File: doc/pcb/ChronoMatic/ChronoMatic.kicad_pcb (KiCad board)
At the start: 2 copper layers, 73 x 73.1 mm, 24 parts, among them Q1 Q_Photo_NPN, U1 STM32F030F4Px, Y1 7.3728

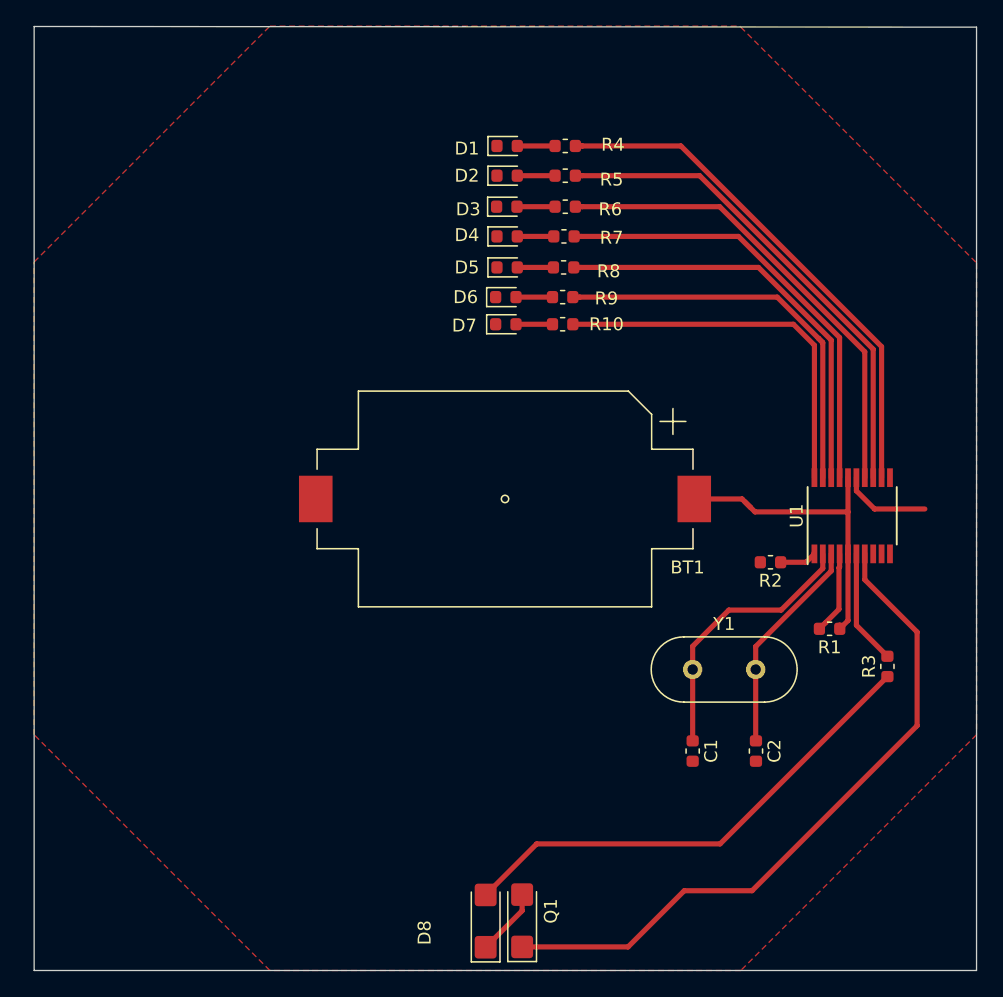
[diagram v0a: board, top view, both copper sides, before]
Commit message: new design
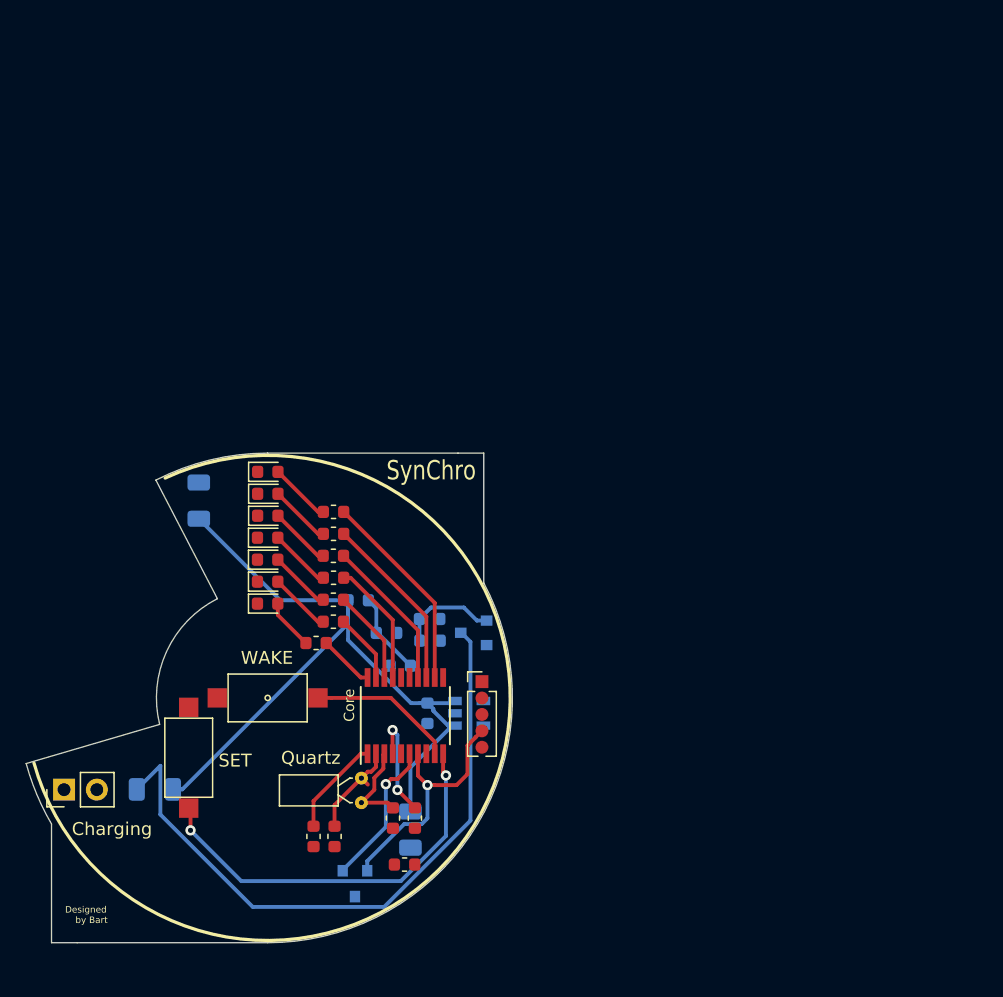
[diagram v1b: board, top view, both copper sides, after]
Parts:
- removed D8: LED, LED_SMD:LED_1806_4516Metric_Castellated
- removed Y1: 7.3728, Crystal:Crystal_HC49-U_Vertical
- added   : Conn_01x05_Female, Connector_PinHeader_1.27mm:PinHeader_1x05_P1.27mm_Vertical, F.Cu at (235.7, 115.0)
- added BT2: Battery_Cell, Resistor_SMD:R_1206_3216Metric, B.Cu at (230.2, 126.5)
- added C3: 10p, Capacitor_SMD:C_0603_1608Metric, F.Cu at (224.3, 127.0)
- added C4: 10p, Capacitor_SMD:C_0603_1608Metric, F.Cu at (228.8, 125.6)
- added C5: 2.2u, Capacitor_SMD:C_0603_1608Metric, B.Cu at (228.3, 111.3)
- added Charging: Charging port, Connector_PinHeader_2.54mm:PinHeader_1x02_P2.54mm_Vertical, F.Cu at (203.3, 123.4)
- added Core: STM32F041F6Px, Package_SO:TSSOP-20_4.4x6.5mm_P0.65mm, F.Cu at (229.8, 117.7)
- added M1: Motor_DC, Resistor_SMD:R_1206_3216Metric, B.Cu at (210.4, 123.4)
- added Quartz: 32.768, Crystal:Crystal_DS26_D2.0mm_L6.0mm_Horizontal, F.Cu at (226.4, 122.5)
- added R11: 15k, Resistor_SMD:R_0603_1608Metric, B.Cu at (231.6, 110.2)
- added R12: 100k, Resistor_SMD:R_0603_1608Metric, B.Cu at (226.1, 108.7)
- added R13: 100k, Resistor_SMD:R_0603_1608Metric, B.Cu at (229.4, 113.8)
- added SET: SET, Button_Switch_SMD:SW_SPST_CK_RS282G05A3, F.Cu at (213.0, 120.9)
- added U4: SS311PT, Package_TO_SOT_SMD:SOT-23, B.Cu at (225.9, 130.7)
- added WAKE: WAKE, Button_Switch_SMD:SW_SPST_CK_RS282G05A3, F.Cu at (219.1, 116.3)
- BT1: footprint Battery:BatteryHolder_Keystone_1060_1x2032 -> Resistor_SMD:R_1206_3216Metric; moved to B.Cu
- C1: value 22p -> 100n; moved to B.Cu
- C2: value 22p -> 100n
- Q1: value Q_Photo_NPN -> IRLML0030TR; footprint LED_SMD:LED_1806_4516Metric_Castellated -> Package_TO_SOT_SMD:SOT-23; moved to B.Cu
- R10, R4, R5, R6, R7, R8, R9: value 220R -> 1k
- R3: value 22R -> 220R; moved to B.Cu
- U1: value STM32F030F4Px -> TC1185-3.3VCT8; footprint Package_SO:TSSOP-20_4.4x6.5mm_P0.65mm -> Package_TO_SOT_SMD:SOT-23-5; moved to B.Cu
- moved R2 41.3 mm to (222.7, 127.0), turned to 270 degrees
- moved R3 35.5 mm to (231.7, 111.9), turned to 0 degrees
- moved R1 35.3 mm to (230.5, 125.6), turned to 90 degrees
- moved R4 33.5 mm to (224.2, 101.9)
- moved U1 33.4 mm to (234.7, 117.5), turned to 0 degrees
- moved R5 33.0 mm to (224.2, 103.6)
- moved R6 32.4 mm to (224.2, 105.3)
- moved R7 31.9 mm to (224.2, 107.0)
- moved R8 31.3 mm to (224.2, 108.7)
- moved D1 31.3 mm to (219.1, 98.8)
- moved R10 31.2 mm to (222.8, 112.0)
- moved D2 30.8 mm to (219.1, 100.5)
- moved R9 30.8 mm to (224.2, 110.4)
- moved D3 30.2 mm to (219.1, 102.2)
- moved D4 29.8 mm to (219.1, 103.9)
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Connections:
- BT1 pad 1: Vcc -> +5V
- C1 pad 1: Net-(C1-Pad1) -> +5V
- C2 pad 1: Net-(C2-Pad1) -> Vcc
- Q1 pad 1: DIO -> Net-(Q1-Pad1)
- R3 pad 1: Net-(D8-Pad2) -> Net-(Q1-Pad1)
- U1 pad 1: Net-(R2-Pad1) -> +5V
- U1 pad 2: Net-(C1-Pad1) -> GND
- U1 pad 3: Net-(C2-Pad1) -> +5V
- U1 pad 4: RST -> (no net)
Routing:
- net +5V: track 0.00 -> 59.4 mm
- net Net-(M1-Pad2): track 0.00 -> 51.0 mm
- net Net-(D8-Pad2): track 38.1 -> 0.00 mm
- net DIO: track 52.6 -> 19.4 mm, vias 0 -> 1
- net Net-(SW2-Pad1): track 0.00 -> 31.1 mm, vias 0 -> 2
- net Vcc: track 30.9 -> 0.00 mm
- net Net-(R9-Pad2): track 31.7 -> 5.36 mm
- net Net-(R8-Pad2): track 32.9 -> 7.33 mm
- net Net-(R10-Pad2): track 29.6 -> 4.30 mm
- net Net-(R7-Pad2): track 34.6 -> 9.61 mm
- net Net-(R6-Pad2): track 36.8 -> 11.8 mm
- net Net-(R5-Pad2): track 38.6 -> 13.8 mm
- net Net-(R4-Pad2): track 40.3 -> 15.7 mm
- net Net-(C1-Pad1): track 21.0 -> 0.00 mm
- net Net-(C2-Pad1): track 16.9 -> 0.00 mm
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- removed copper zone on F.Cu, net GND
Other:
- board size 73 x 73.1 mm -> 37.6 x 37.9 mm
- board text added: "+"
- board text added: "Designed by Bart"
- board text added: "SynChro"
